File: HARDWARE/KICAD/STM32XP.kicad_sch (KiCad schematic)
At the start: 64 parts, among them J1 USB_C_Receptacle_USB2.0_16P, J2 Micro_SD_Card, J3 Conn_01x20_Socket, J4 Conn_01x20_Socket, J5 Jack-DC, J9 Conn_02x05_Odd_Even, SW1 SW_Push, SW2 SW_Push, SW3 RST, U1 STM32F411RETx, U2 ADS1115IDGS, U3 LM324, U4 AMS1117-3.3, U5 USBLC6-2SC6, U6 OLED 128x64 1.3", Y1 32.768kHz, Y2 8MHz xpF

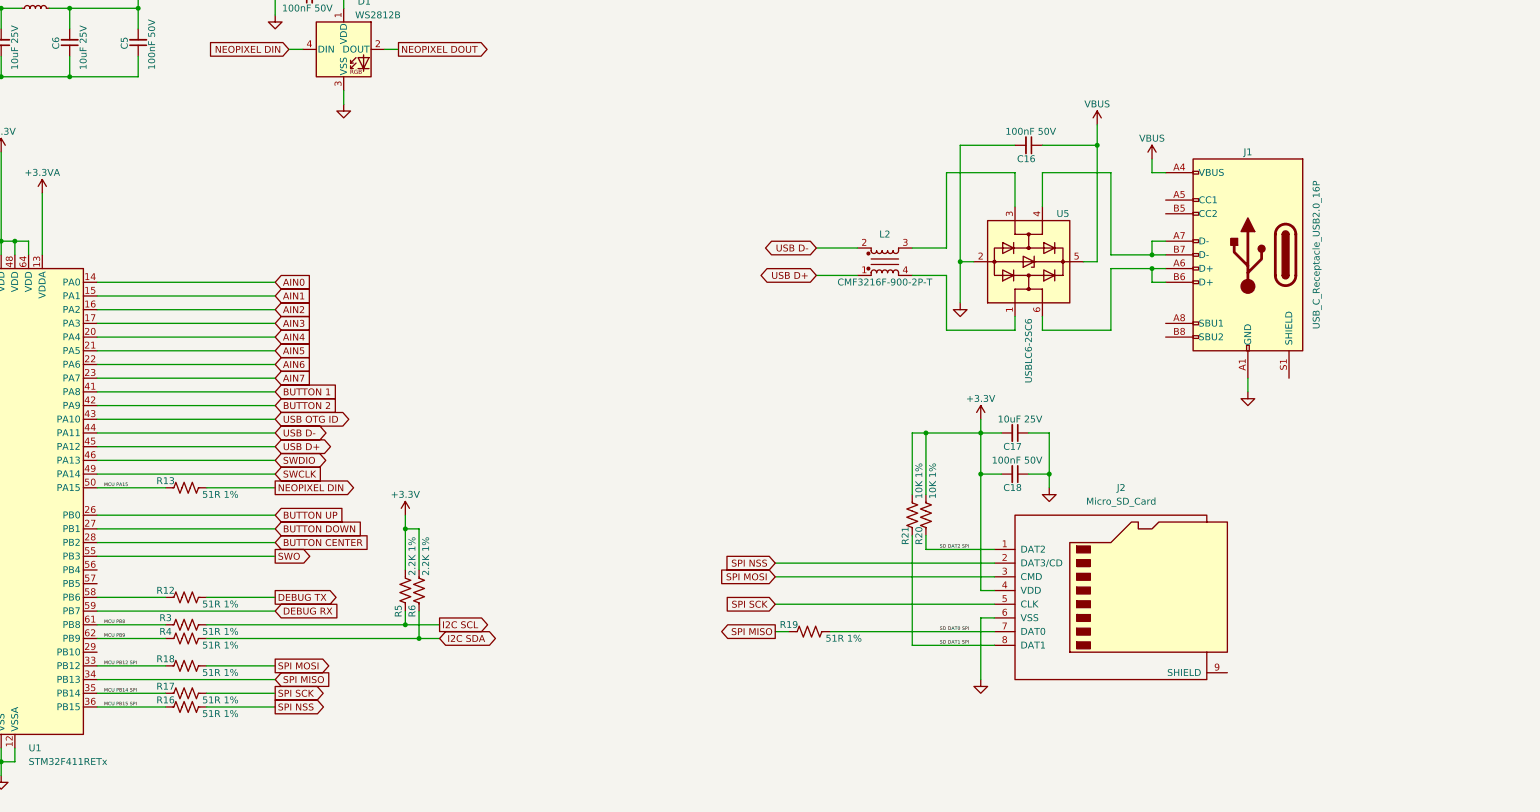
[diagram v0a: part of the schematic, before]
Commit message: Added RGBfunctionality. Corrected SPI connections on schematic and layout.
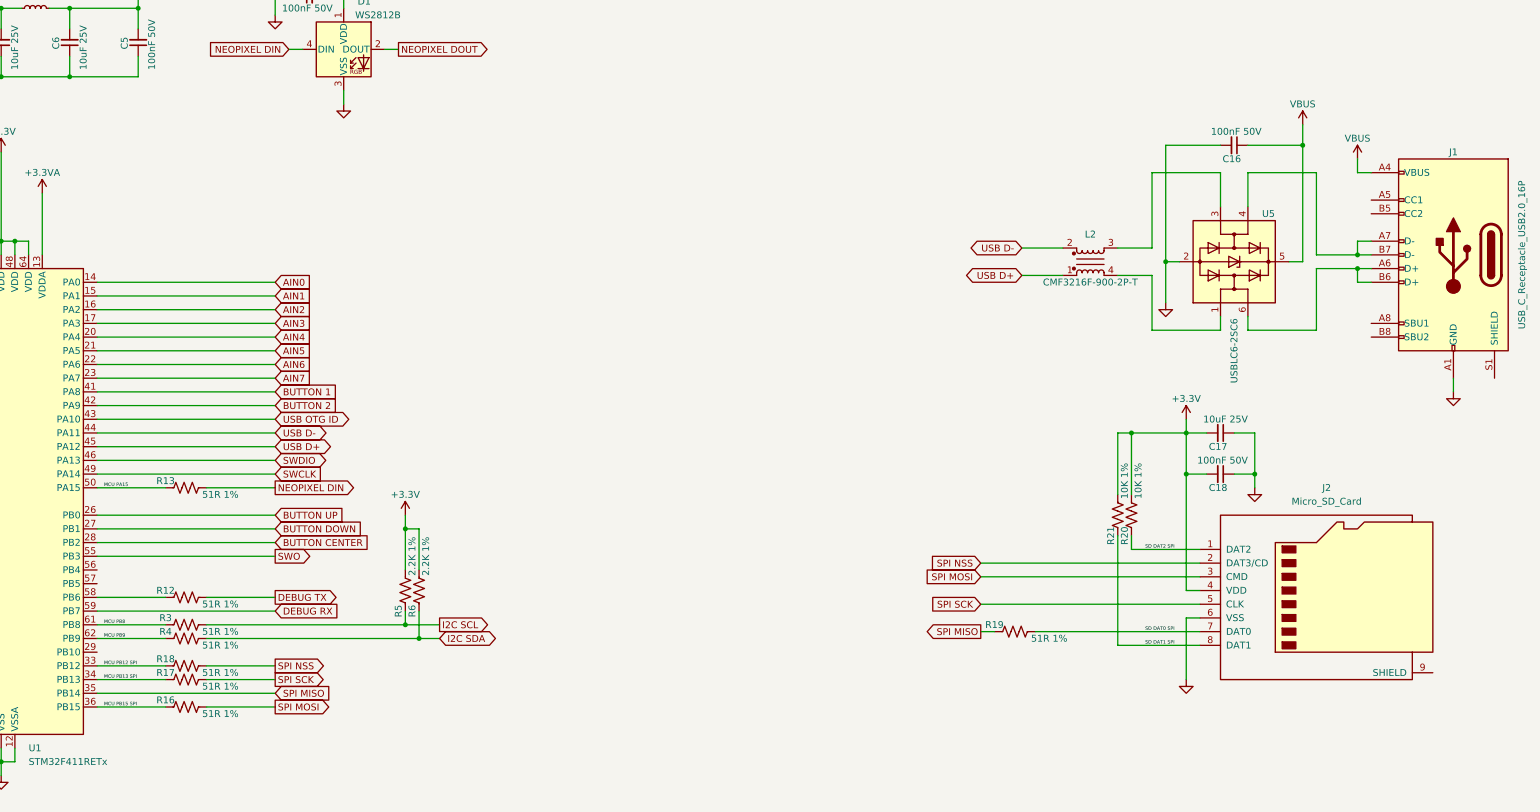
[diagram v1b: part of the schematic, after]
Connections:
- net SPI MISO: now also U1.35 (PB14); no longer U1.34 (PB13)
- net SPI MOSI: now also R16.2; no longer R18.2
- net SPI NSS: now also R18.2; no longer R16.2
- net MCU PB14 SPI renamed MCU PB13 SPI
- net MCU PB13 SPI: now also U1.34 (PB13); no longer U1.35 (PB14)
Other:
- moved on the sheet: C16, C17, C18, J1, J2, L2, R17, R19, R20, R21, U5

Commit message: Added AFE circuit.
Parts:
- added C19, C20, C21, C22, C23, C24, C25, C26, C27, C30: 100nF 50V, Capacitor_SMD:C_0603_1608Metric_Pad1.08x0.95mm_HandSolder, symbol Device:C_Small
- added C28, C29: 10uF 25V, Capacitor_SMD:C_0805_2012Metric_Pad1.18x1.45mm_HandSolder, symbol Device:C_Small
- added R22, R23, R24, R25, R26, R27, R28, R29, R30, R31, R32, R33: 10K 1%, Resistor_SMD:R_0603_1608Metric_Pad0.98x0.95mm_HandSolder, symbol Device:R_US
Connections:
- net +3.3V: no longer U2.8 (VDD)
- net AIN0: now also U2.4 (AIN0), U3.1, U3.2 (-), C20.2, R33.2; no longer J3.3 (Pin_3), U1.14 (PA0)
- net AIN1: now also U2.5 (AIN1), U3.6 (-), U3.7, C21.2, R32.2; no longer J3.4 (Pin_4), U1.15 (PA1)
- net AIN2: now also U2.6 (AIN2), U3.8, U3.9 (-), C23.2, R31.2; no longer J3.5 (Pin_5), U1.16 (PA2)
- net AIN3: now also U2.7 (AIN3), U3.13 (-), U3.14, C25.2, R30.2; no longer J3.6 (Pin_6), U1.17 (PA3)
- net GND: now also J9.10 (Pin_10), J9.2 (Pin_2), J9.4 (Pin_4), J9.5 (Pin_5), J9.6 (Pin_6), J9.8 (Pin_8), U2.1 (ADDR), U3.11 (V-), C19.1, C22.1, C24.1, C26.1, C27.1, C28.1, C29.1, C30.1, R30.1, R31.1, R32.1, R33.1
- net at U3.5 (+): now also C22.2, R25.2
- net at U3.10 (+): now also C24.2, R27.2
- net +5VA: now reaches U3.4 (V+)
- net +5VA: now also U2.8 (VDD), C27.2, C28.2, C29.2, C30.2
- net at U3.3 (+): now also C19.2, R22.2
- net A0: now reaches J9.1 (Pin_1)
- net A0: now also R23.1
- net A1: now reaches J9.3 (Pin_3)
- net A1: now also R24.1
- net A2: now reaches J9.7 (Pin_7)
- net A2: now also R26.1
- net A3: now reaches J9.9 (Pin_9)
- net A3: now also R28.1
- net at U3.12 (+): now also C26.2, R29.2
- net AIN4 renamed PA4
- net AIN5 renamed PA5
- net AIN6 renamed PA6
- net AIN7 renamed PA7
- new net: C20.1, R22.1, R23.2
- new net: C25.1, R28.2, R29.1
- new net: C23.1, R26.2, R27.1
- new net: C21.1, R24.2, R25.1
- new net PA0: J3.3 (Pin_3), U1.14 (PA0)
- new net PA1: J3.4 (Pin_4), U1.15 (PA1)
- new net PA2: J3.5 (Pin_5), U1.16 (PA2)
- new net PA3: J3.6 (Pin_6), U1.17 (PA3)
- no-connect marks 0 -> 1
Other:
- moved on the sheet: J9, U2, U3A, U3B, U3C, U3D, U3E

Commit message: Added PWM outputs from MCU; added directional buttons; added part of buzzer circuit.
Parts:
- added C31: 10uF 25V, Capacitor_SMD:C_0805_2012Metric_Pad1.18x1.45mm_HandSolder, symbol Device:C_Small
- added D2: ESDA6V1-5SC6, Package_TO_SOT_SMD:SOT-23-6, symbol Power_Protection:ESDA6V1-5SC6
- added LS1: Speaker_Crystal, symbol Device:Speaker_Crystal
- added Q1: MMBT3904, Package_TO_SOT_SMD:SOT-23, symbol Transistor_BJT:MMBT3904
- added R34, R35, R36, R37, R38: 10K 1%, Resistor_SMD:R_0603_1608Metric_Pad0.98x0.95mm_HandSolder, symbol Device:R_US
- added SW4, SW5, SW6, SW7, SW8: SW_Push, Button_Switch_SMD:SW_SPST_CK_KXT3, symbol Switch:SW_Push
- added U7: AMS1117-5.0, Package_TO_SOT_SMD:SOT-223-3_TabPin2, symbol Regulator_Linear:AMS1117-5.0
- R30, R31, R32, R33: value 10K 1% -> 51R 1%
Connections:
- net +3.3V: now also R34.2, R35.2, R36.2, R37.2, R38.2
- net +5VA: now also C31.2, U7.2 (VO)
- net A0: now also D2.1 (IO1)
- net A1: now also D2.3 (IO2)
- net AIN0: no longer R33.2
- net AIN1: no longer R32.2
- net AIN2: no longer R31.2
- net AIN3: no longer R30.2
- net BUTTON CENTER: now also R38.1, SW8.2
- net BUTTON DOWN: now also R35.1, SW5.2
- net BUTTON LEFT: now also R36.1, SW6.2
- net BUTTON RIGHT: now also R37.1, SW7.2
- net BUTTON UP: now also R34.1, SW4.2
- net GND: now also C31.1, SW4.1, SW5.1, SW6.1, SW7.1, SW8.1, U7.1 (GND); no longer R30.1, R31.1, R32.1, R33.1
- net at U1.37 (PC6): now also R30.2
- net at U1.38 (PC7): now also R31.2
- net at U1.39 (PC8): now also R32.2
- net at U1.40 (PC9): now also R33.2
- net +9V: now reaches U4.3 (VI)
- net +9V: now also U7.3 (VI)
- new net TIM3 CH1: R30.1
- new net TIM3 CH2: R31.1
- new net TIM3 CH3: R32.1
- new net TIM3 CH4: R33.1
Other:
- moved on the sheet: C12, C27, C28, J5, U2, U4

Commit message: Added sheets and organized schematic; added DC-DC Boost Converter; added connections to headers; general improvements on schematic and layout.
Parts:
- removed BT1: Battery_Cell, Battery:BatteryHolder_Multicomp_BC-2001_1x2032, symbol Device:Battery_Cell
- removed C1, C13, C14, C15, C16, C18, C19, C2, C20, C21, C22, C23, C24, C25, C26, C27, C3, C30, C4, C5, C8: 100nF 50V, Capacitor_SMD:C_0603_1608Metric_Pad1.08x0.95mm_HandSolder, symbol Device:C_Small
- removed C10, C9: 10pF 50V, Capacitor_SMD:C_0603_1608Metric_Pad1.08x0.95mm_HandSolder, symbol Device:C_Small
- removed C11, C12, C17, C28, C29, C31, C6, C7: 10uF 25V, Capacitor_SMD:C_0805_2012Metric_Pad1.18x1.45mm_HandSolder, symbol Device:C_Small
- removed D1: WS2812B, LED_SMD:LED_WS2812B_PLCC4_5.0x5.0mm_P3.2mm, symbol LED:WS2812B
- removed D2: ESDA6V1-5SC6, Package_TO_SOT_SMD:SOT-23-6, symbol Power_Protection:ESDA6V1-5SC6
- removed H1, H2, H3, H4: MountingHole, MountingHole:MountingHole_3.2mm_M3, symbol Mechanical:MountingHole
- removed J1: USB_C_Receptacle_USB2.0_16P, Connector_USB:USB_C_Receptacle_G-Switch_GT-USB-7010ASV, symbol Connector:USB_C_Receptacle_USB2.0_16P
- removed J2: Micro_SD_Card, Connector_Card:microSD_HC_Wuerth_693072010801, symbol Connector:Micro_SD_Card
- removed J3, J4: Conn_01x20_Socket, Connector_PinSocket_2.54mm:PinSocket_1x20_P2.54mm_Horizontal, symbol Connector:Conn_01x20_Socket
- removed J5: Jack-DC, Connector_BarrelJack:BarrelJack_GCT_DCJ200-10-A_Horizontal, symbol Connector:Barrel_Jack_Switch
- removed J9: Conn_02x05_Odd_Even, Connector_PinSocket_2.54mm:PinSocket_2x05_P2.54mm_Horizontal, symbol Connector_Generic:Conn_02x05_Odd_Even
- removed L1: L_Small, Inductor_SMD:L_0603_1608Metric_Pad1.05x0.95mm_HandSolder, symbol Device:L_Small
- removed L2: CMF3216F-900-2P-T, Inductor_SMD:L_CommonModeChoke_TDK_ACM2520-2P, symbol Device:EMI_Filter_LL_1423
- removed LS1: Speaker_Crystal, symbol Device:Speaker_Crystal
- removed Q1: MMBT3904, Package_TO_SOT_SMD:SOT-23, symbol Transistor_BJT:MMBT3904
- removed R1, R10, R14, R15, R20, R21, R22, R23, R24, R25, R26, R27, R28, R29, R34, R35, R36, R37, R38: 10K 1%, Resistor_SMD:R_0603_1608Metric_Pad0.98x0.95mm_HandSolder, symbol Device:R_US
- removed R11, R12, R13, R16, R17, R18, R19, R3, R30, R31, R32, R33, R4, R7, R8, R9: 51R 1%, Resistor_SMD:R_0603_1608Metric_Pad0.98x0.95mm_HandSolder, symbol Device:R_US
- removed R2: 0R, Resistor_SMD:R_0603_1608Metric_Pad0.98x0.95mm_HandSolder, symbol Device:R_US
- removed R5, R6: 2.2K 1%, Resistor_SMD:R_0603_1608Metric_Pad0.98x0.95mm_HandSolder, symbol Device:R_US
- removed SW1, SW2, SW4, SW5, SW6, SW7, SW8: SW_Push, Button_Switch_SMD:SW_SPST_CK_KXT3, symbol Switch:SW_Push
- removed SW3: RST, Button_Switch_SMD:SW_SPST_CK_KXT3, symbol Switch:SW_Push
- removed U1: STM32F411RETx, Package_QFP:LQFP-64_10x10mm_P0.5mm, symbol MCU_ST_STM32F4:STM32F411RETx
- removed U2: ADS1115IDGS, Package_SO:TSSOP-10_3x3mm_P0.5mm, symbol Analog_ADC:ADS1115IDGS
- removed U3: LM324, Package_SO:TSSOP-14_4.4x5mm_P0.65mm, symbol Amplifier_Operational:LM324
- removed U4: AMS1117-3.3, Package_TO_SOT_SMD:SOT-223-3_TabPin2, symbol Regulator_Linear:AMS1117-3.3
- removed U5: USBLC6-2SC6, Package_TO_SOT_SMD:SOT-23-6, symbol Power_Protection:USBLC6-2SC6
- removed U6: OLED 128x64 1.3", STM32XP:OLED 128x64 1.3in, symbol STM32XP:OLED_128x64
- removed U7: AMS1117-5.0, Package_TO_SOT_SMD:SOT-223-3_TabPin2, symbol Regulator_Linear:AMS1117-5.0
- removed Y1: 32.768kHz, Crystal:Crystal_SMD_G8-2Pin_3.2x1.5mm_HandSoldering, symbol Device:Crystal
- removed Y2: 8MHz xpF, Crystal:Crystal_SMD_EuroQuartz_MT-4Pin_3.2x2.5mm_HandSoldering, symbol Device:Crystal_GND24
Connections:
- no-connect marks 1 -> 0
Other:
- added sheet ANALOG (ANALOG.kicad_sch)
- added sheet INTERFACE (INTERFACE.kicad_sch)
- added sheet IO (IO.kicad_sch)
- added sheet MCU (MCU.kicad_sch)
- added sheet MECHANICAL (MECHANICAL.kicad_sch)
- added sheet POWER (POWER.kicad_sch)
